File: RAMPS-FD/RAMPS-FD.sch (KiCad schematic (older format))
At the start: 7 parts, among them M101 LOGO_OSHW, M102 PCB_GREEN_RMC, P106 CONN_3X2, SW101 SW_PUSH

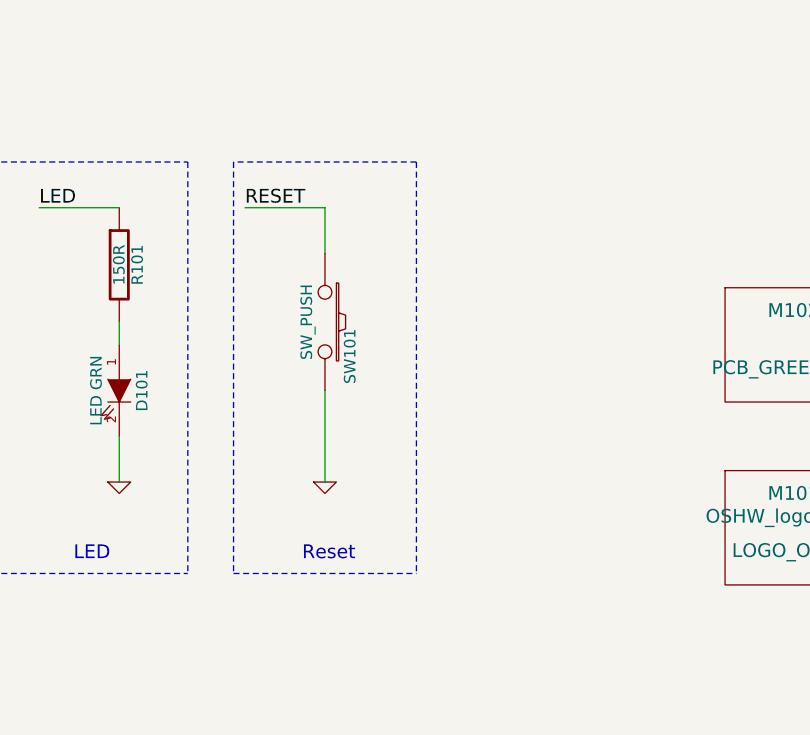
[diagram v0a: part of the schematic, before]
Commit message: RAMPS-FD: version 1 Rev A
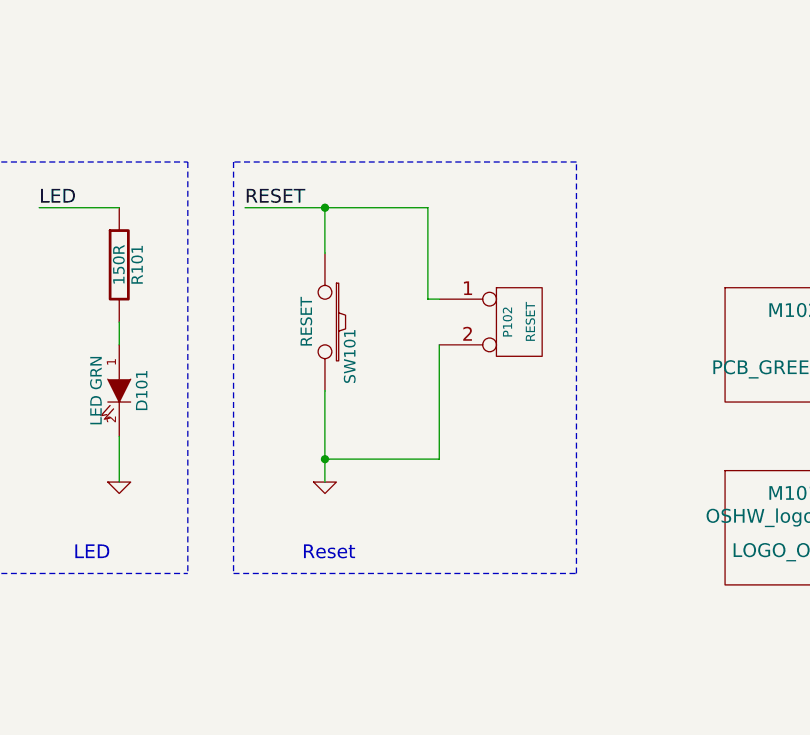
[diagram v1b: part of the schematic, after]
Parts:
- added P102: RESET, symbol CONN_2
- SW101: value SW_PUSH -> RESET
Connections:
- net GND: now also P102.2 (PM)
- net RESET: now also P102.1 (P1)
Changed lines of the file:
@@
 Sheet 1 9
 Title "RAMPS-FD (RAMPS for Arduino Due)"
-Date "26 sep 2013"
+Date "3 oct 2013"
 Rev "0.2"
 Comp ""
@@
 P 8650 5100
 F 0 "SW101" H 8800 5210 50  0000 C CNN
-F 1 "SW_PUSH" H 8650 5020 50  0000 C CNN
+F 1 "RESET" H 8650 5020 50  0000 C CNN
 F 2 "" H 8650 5100 60  0001 C CNN
 F 3 "" H 8650 5100 60  0001 C CNN
@@
 	4750 1850 4100 1850
 Wire Notes Line
-	9050 4400 9050 6200
-Wire Notes Line
-	9050 4400 8250 4400
+	9750 6200 9750 4400
+Wire Notes Line
+	9750 4400 8250 4400
 Wire Wire Line
 	1000 5400 2200 5400
@@
 	8250 4400 8250 6200
 Wire Notes Line
-	8250 6200 9050 6200
+	8250 6200 9750 6200
 Wire Notes Line
 	7150 6200 7150 4400
@@
 	1450 6050 2200 6050
 Wire Wire Line
-	8300 4600 8650 4600
+	8300 4600 9100 4600
 Wire Wire Line
 	8650 4600 8650 4800
@@
 Text GLabel 4750 1650 2    50   Output ~ 0
 D13
+$Comp
+L CONN_2 P102
+U 1 1 52475D81
+P 9500 5100
+F 0 "P102" V 9450 5100 40  0000 C CNN
+F 1 "RESET" V 9550 5100 40  0000 C CNN
+F 2 "" H 9500 5100 60  0000 C CNN
+F 3 "" H 9500 5100 60  0000 C CNN
+	1    9500 5100
+	1    0    0    -1
+$EndComp
+Wire Wire Line
+	9100 4600 9100 5000
+Wire Wire Line
+	9100 5000 9150 5000
+Connection ~ 8650 4600
+Wire Wire Line
+	9150 5200 9150 5700
+Wire Wire Line
+	9150 5700 8650 5700
+Connection ~ 8650 5700
 $EndSCHEMATC
